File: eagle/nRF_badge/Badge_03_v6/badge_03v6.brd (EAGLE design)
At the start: 30 x 70 mm, 43 parts, among them U1 LIS2DH12, U2 LP2985LV, U3 MCP6231, U5 M95M02, Y1 32768Hz

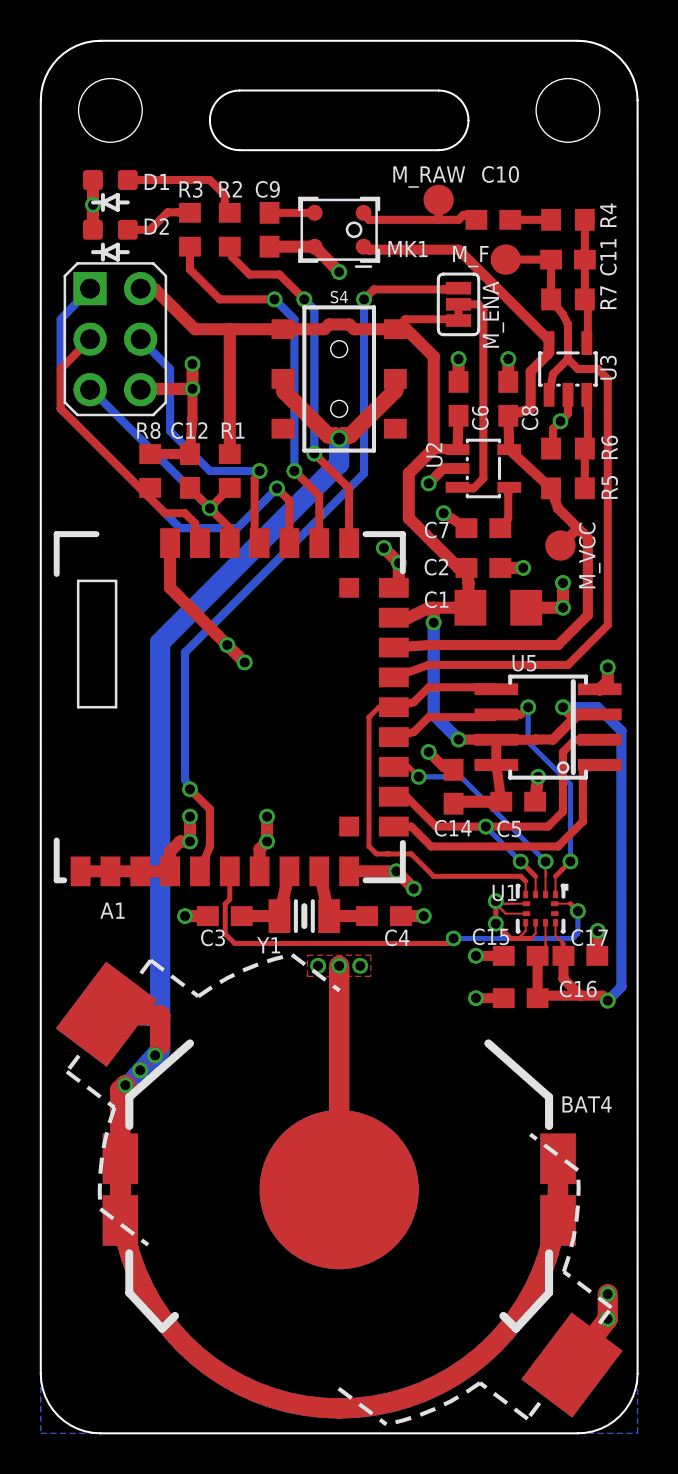
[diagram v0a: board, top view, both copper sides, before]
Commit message: Fix for issues generated in last commit, updated library
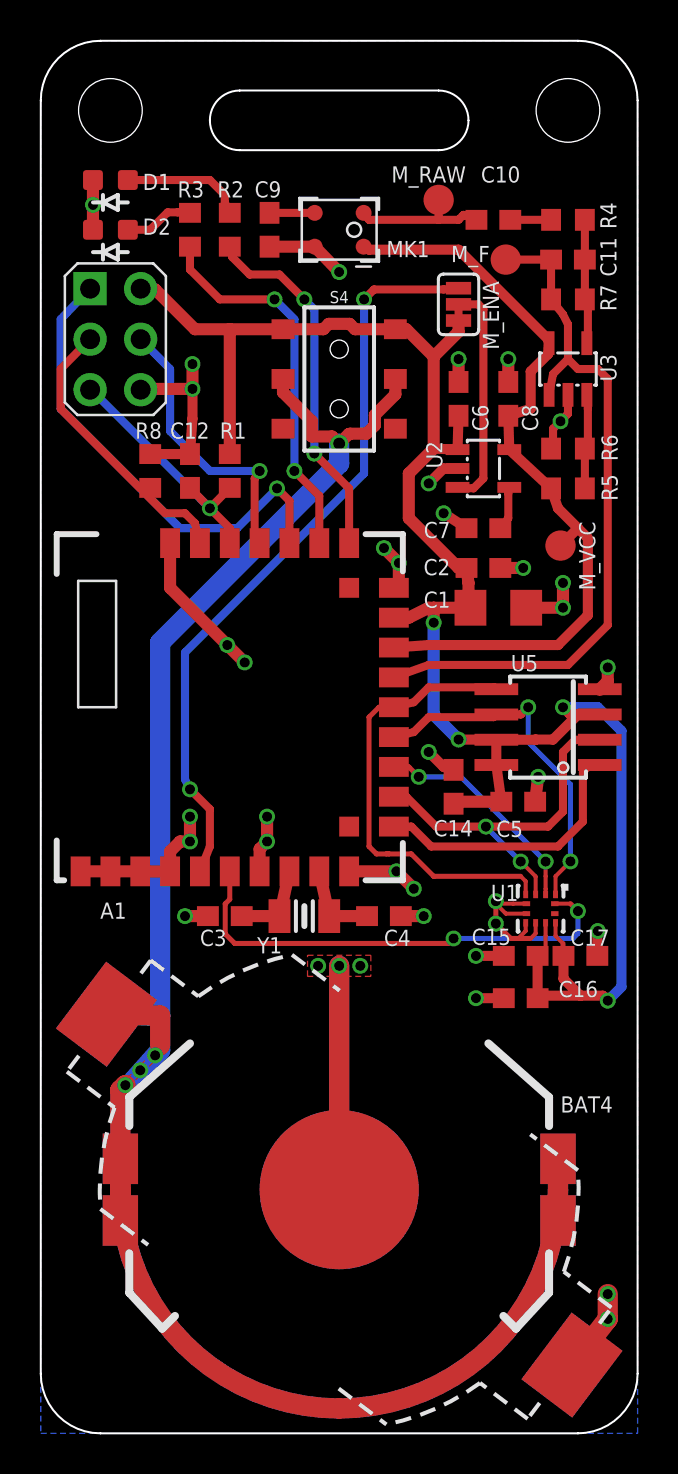
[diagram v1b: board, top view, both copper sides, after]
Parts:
- U1: value LIS2DH12 -> LIS2DH12"; device st-microelectronics_modified:LGA12-TN0018-COMPLIANT -> Badge:LGA12-TN0018-COMPLIANT
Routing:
- net VCC: track 98.9 -> 97.9 mm
- net VBATT: track 140.2 -> 140.7 mm
